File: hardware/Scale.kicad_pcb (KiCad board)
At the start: 2 copper layers, 45 x 45 mm, 111 parts, among them J1 Load Cell Connector, J2 GPIO, J3 RS232, J4 DebugEdge_02x03, J5 Display Connector, J7 12401610E4#2A, Q1 DMG2307L, Q2 DMG2307L, Q3 BSD235N, SW1 RESET, U1 STM32G070CBTx_u, U10 MCP6001-OT, U2 MCP3562R-E/ST, U3 MCP6N11-010, U4 MCP4542, U7 AP9101CK, U8 MIC5504-3.3YM5, U9 MCP6001-OT, X1 KC2520Z

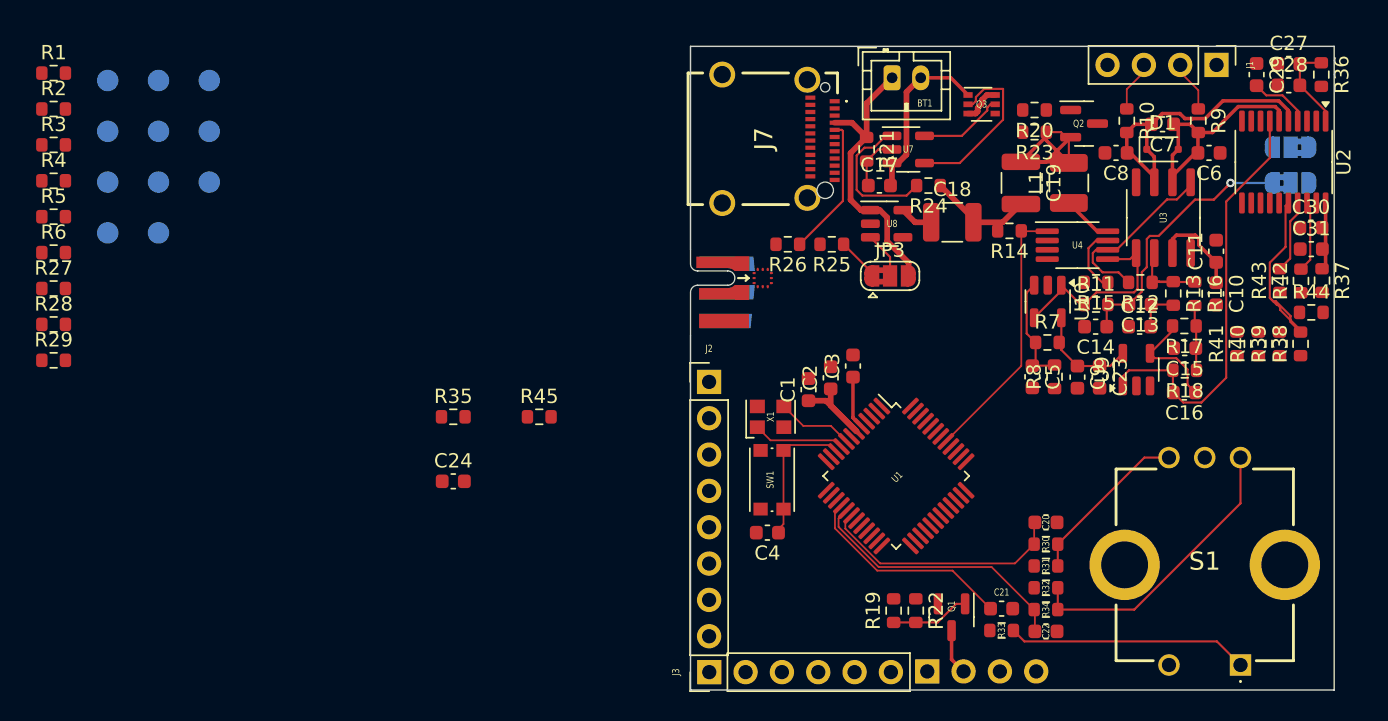
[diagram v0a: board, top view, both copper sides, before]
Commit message: Some more routing
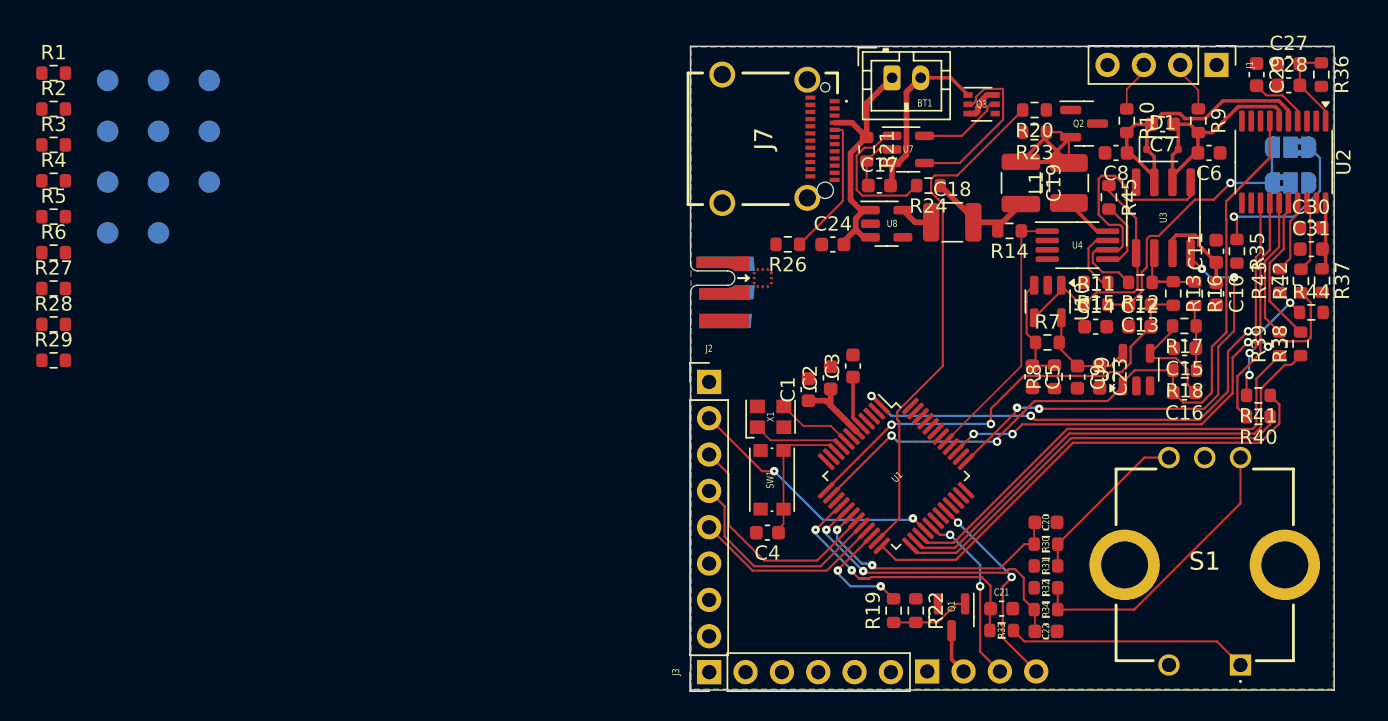
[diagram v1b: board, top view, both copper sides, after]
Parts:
- removed JP3: SolderJumper_3_Bridged12, Jumper:SolderJumper-3_P1.3mm_Bridged2Bar12_RoundedPad1.0x1.5mm
- removed R25: 100K, Resistor_SMD:R_0603_1608Metric
- moved R35 56.0 mm to (151.4, 60.8), turned to -90 degrees
- moved R45 42.7 mm to (142.5, 57.0), turned to -90 degrees
- moved C24 31.3 mm to (123.2, 60.3)
- moved R40 5.10 mm to (152.9, 72.3), turned to 180 degrees
- moved R41 3.90 mm to (152.9, 70.8), turned to 180 degrees
- turned C14 to 0 degrees
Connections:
- U1 pad 3: /MCU/LDO_EN -> unconnected-(U1C-PC15-OSC32_OUT(PC15)/RCC_OSC32_EN/RCC_OSC32_OUT/RCC_OSC_EN/TIM15_BK-Pad3)
- U1 pad 4: +BATT -> +3.3VA
- U8 pad 3: Net-(JP3-C) -> +BATT
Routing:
- net /ADC/ADC_IRQ: track 0.00 -> 38.1 mm, vias 0 -> 4
- net /MCU/BRIDGE_ENABLE: track 0.00 -> 36.1 mm
- net /ADC/~{SS}: track 0.00 -> 34.4 mm
- net /ADC/MISO: track 0.00 -> 34.3 mm
- net /ADC/ADC_MCLK: track 0.00 -> 33.3 mm, vias 0 -> 4
- net /ADC/MOSI: track 0.00 -> 32.6 mm
- net /Instrumentation Amplifier/INA_ENABLE: track 0.00 -> 32.3 mm, vias 0 -> 4
- net /ADC/CLK: track 0.00 -> 29.6 mm
- net /Instrumentation Amplifier/INA_OUT_FILTERED_PASSIVE: track 3.03 -> 31.7 mm, vias 0 -> 2
- net /ADC/INA_OUT_FILTERED_ACTIVE: track 29.8 -> 57.8 mm, vias 0 -> 2
- net /MCU/GPIO_PA8: track 0.00 -> 18.5 mm, vias 0 -> 2
- net /MCU/GPIO_PB0: track 0.00 -> 16.6 mm
- net Net-(U2-SCK): track 0.00 -> 16.2 mm
- net /MCU/GPIO_PB1: track 0.00 -> 15.3 mm
- net /Display/SDA: track 0.00 -> 14.4 mm, vias 0 -> 2
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- added copper zone on B.Cu, net GND
- added copper zone on F.Cu, net GND
